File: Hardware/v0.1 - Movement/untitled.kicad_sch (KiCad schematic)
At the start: 32 parts, among them J7 Motor (left), J8 Motor (right), Q10 IRF540N, Q11 IRF9540N, Q12 IRF540N, Q13 IRF540N, Q14 IRF9540N, Q15 IRF540N, Q3 IRF540N, Q5 IRF9540N, Q6 IRF540N, Q7 IRF540N, Q8 IRF9540N, Q9 IRF540N

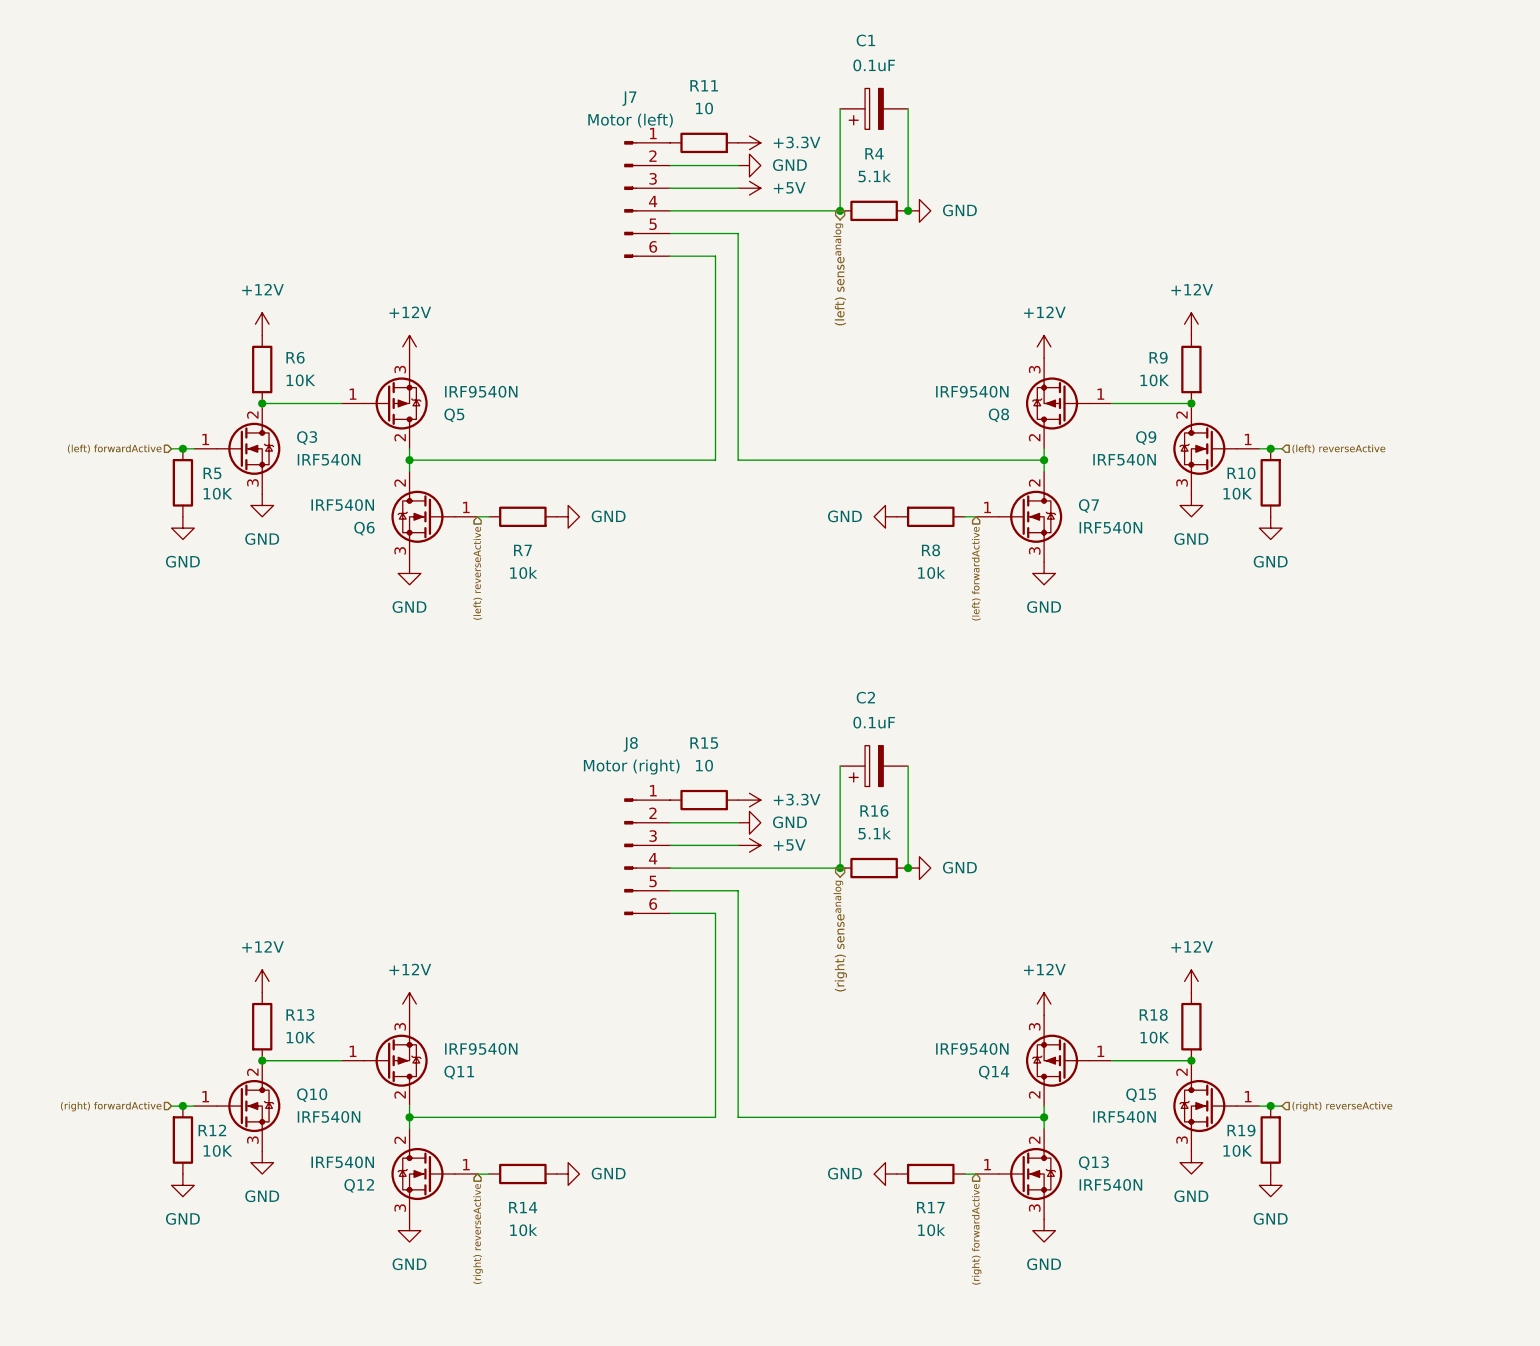
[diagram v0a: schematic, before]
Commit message: added session 17
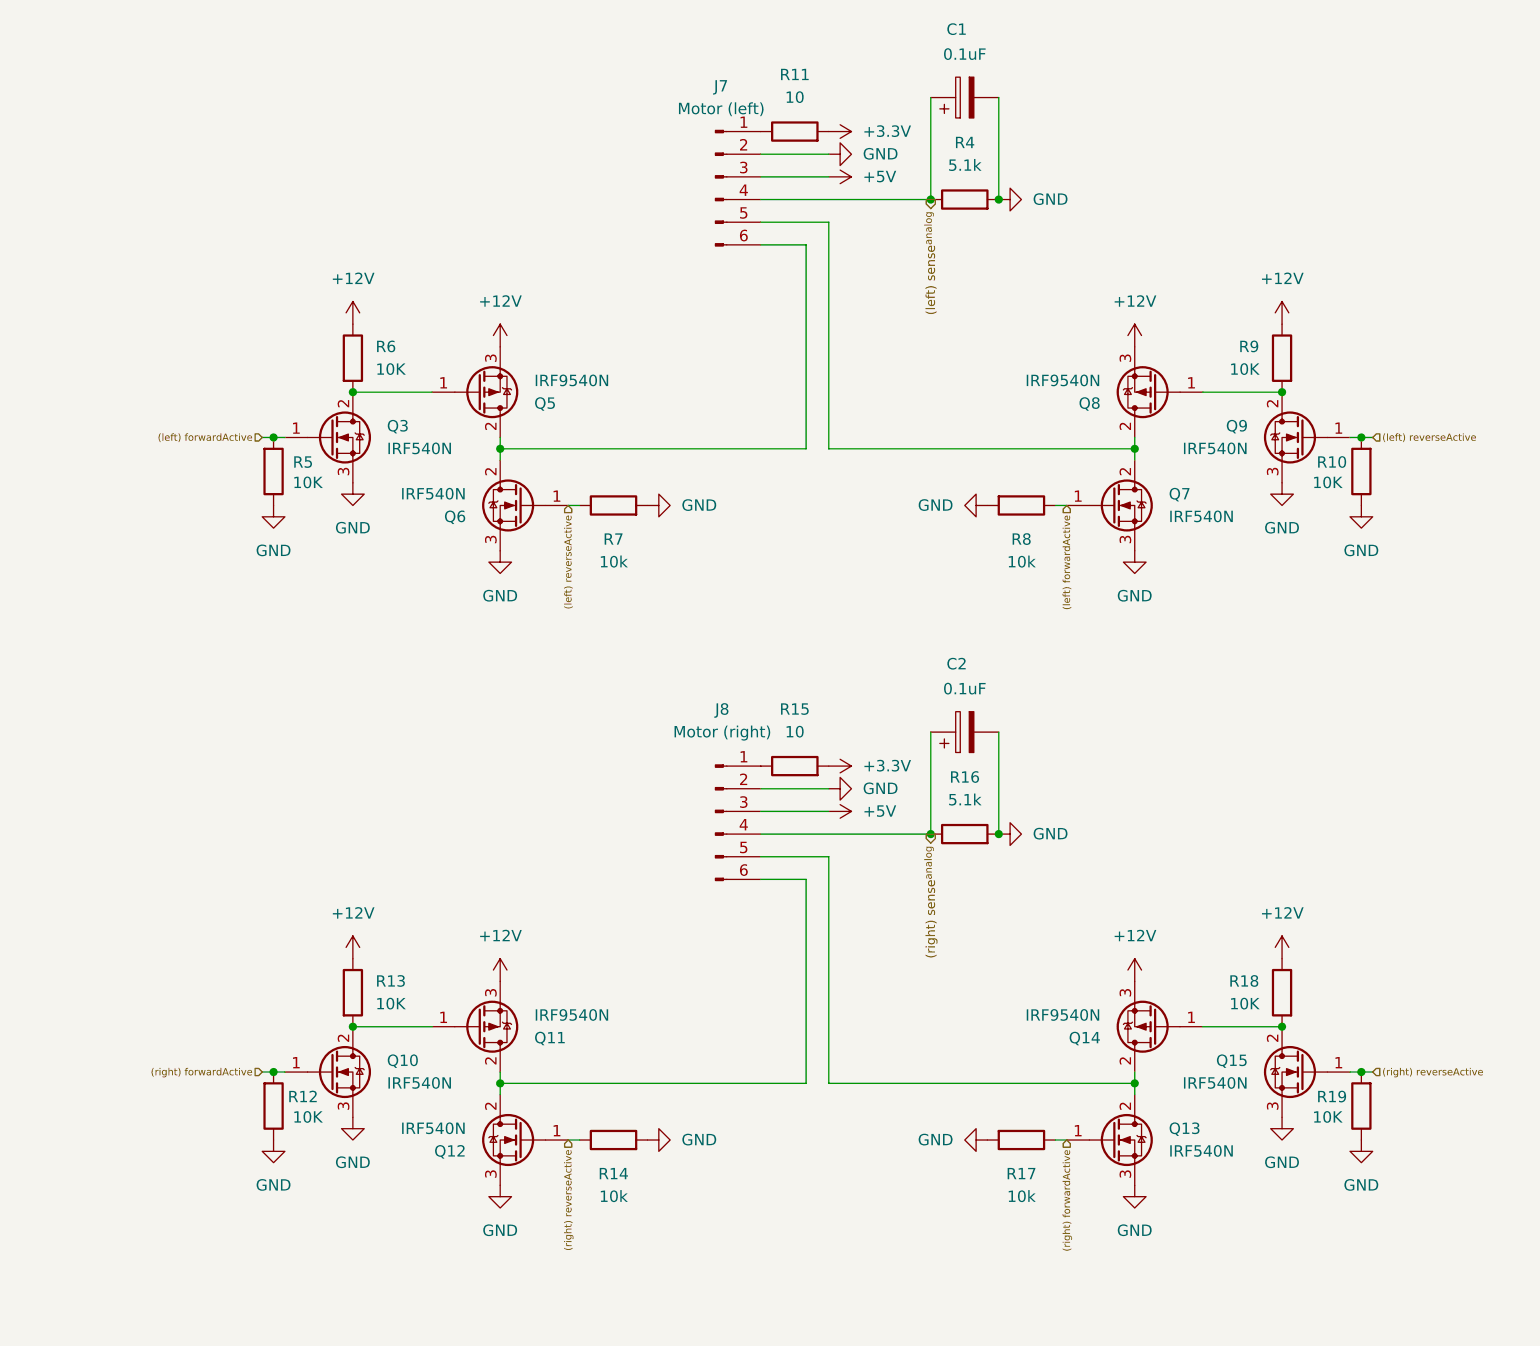
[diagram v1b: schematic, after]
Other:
- company: (none) -> Karl Wünsche
- title: (none) -> Motor Circuit
- moved on the sheet: C1, C2, J7, J8, Q10, Q11, Q12, Q13, Q14, Q15, Q3, Q5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
